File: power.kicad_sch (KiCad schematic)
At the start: 11 parts, among them U3 MAX20356AEWY+T

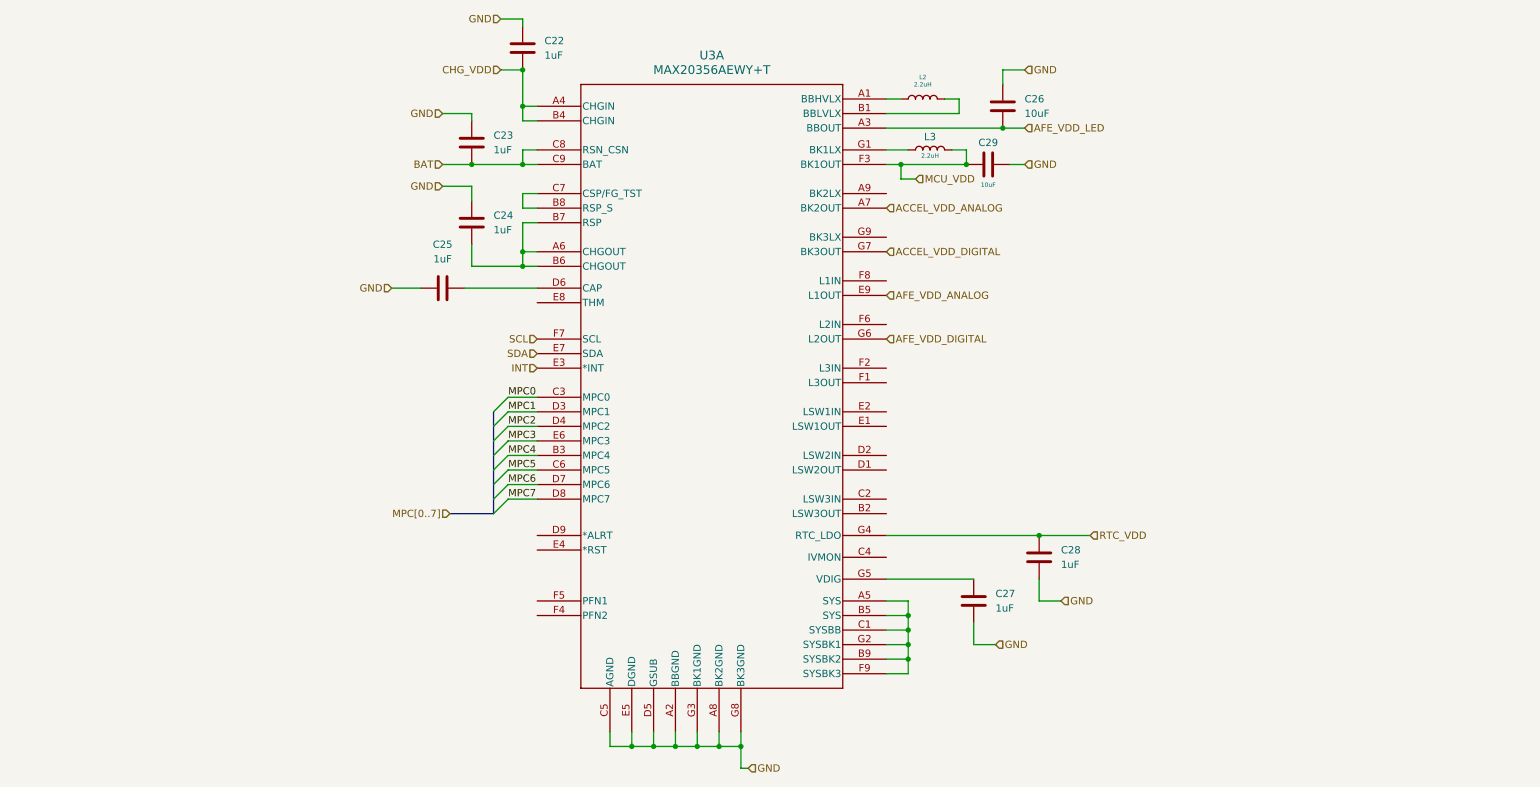
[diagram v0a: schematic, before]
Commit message: inital routing
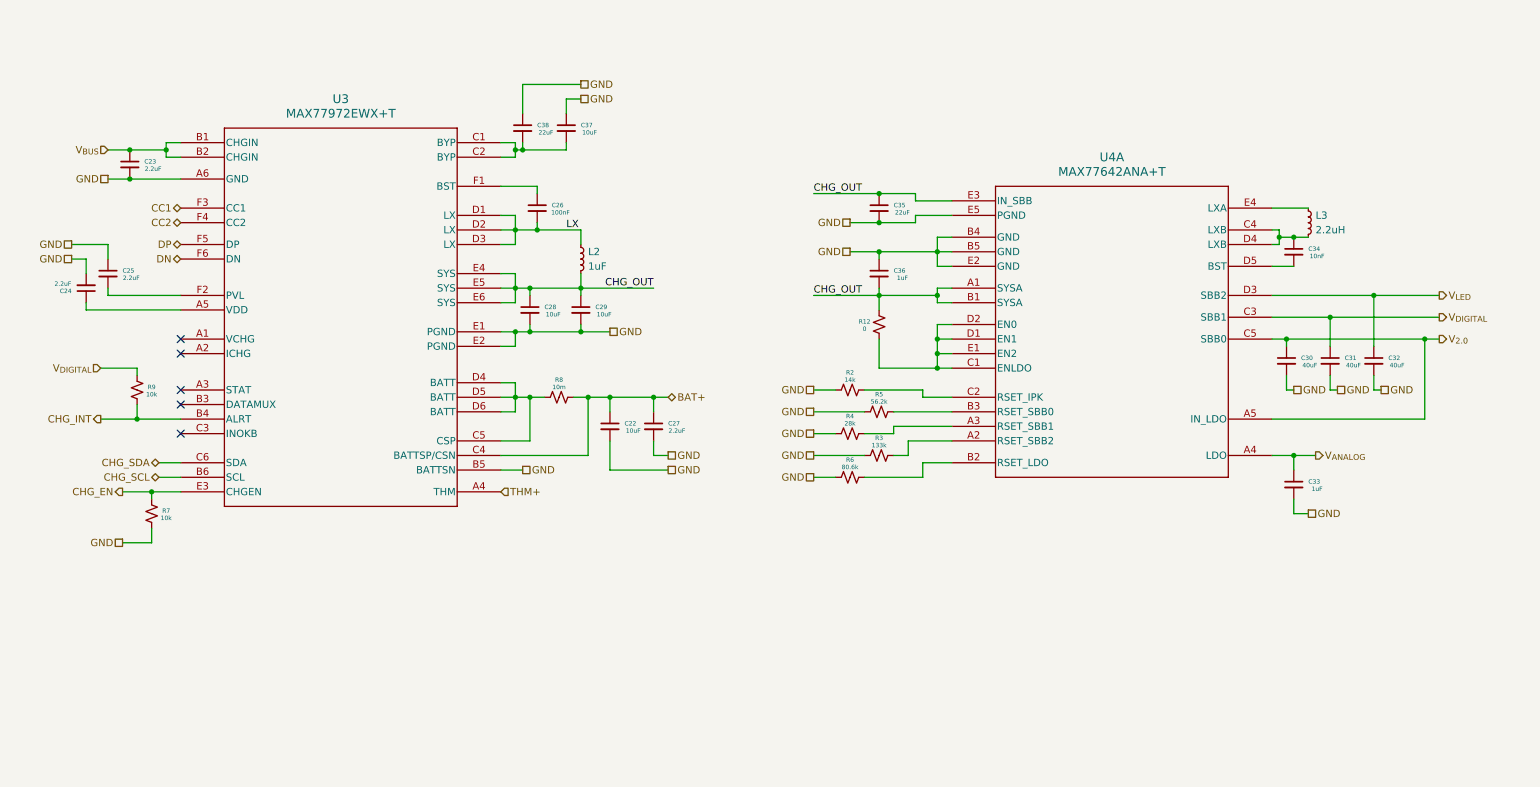
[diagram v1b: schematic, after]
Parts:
- removed C22, C23, C24, C25, C27, C28: 1uF, symbol Device:C
- removed C26, C29: 10uF, symbol Device:C
- removed L2, L3: 2.2uH, symbol Device:L
- removed U3: MAX20356AEWY+T, 21-100616_W633A4+1_ADI, symbol ProjectSymbols:MAX20356AEWY+T
- added C22, C28, C29, C37: 10uF, Capacitor_SMD:C_0402_1005Metric, symbol Device:C_Small
- added C23, C24, C25, C27: 2.2uF, Capacitor_SMD:C_0201_0603Metric, symbol Device:C_Small
- added C26: 100nF, Capacitor_SMD:C_01005_0402Metric, symbol Device:C_Small
- added C30, C31, C32: 40uF, Capacitor_SMD:C_0805_2012Metric, symbol Device:C_Small
- added C33, C36: 1uF, Capacitor_SMD:C_0201_0603Metric, symbol Device:C_Small
- added C34: 10nF, Capacitor_SMD:C_01005_0402Metric, symbol Device:C_Small
- added C35, C38: 22uF, Capacitor_SMD:C_0402_1005Metric, symbol Device:C_Small
- added L2: 1uF, Inductor_SMD:L_0805_2012Metric, symbol Device:L_Small
- added L3: 2.2uH, Inductor_SMD:L_1210_3225Metric, symbol Device:L_Small
- added R12: 0, Resistor_SMD:R_0603_1608Metric, symbol Device:R_Small_US
- added R2: 14k, Resistor_SMD:R_0603_1608Metric, symbol Device:R_Small_US
- added R3: 133k, Resistor_SMD:R_0603_1608Metric, symbol Device:R_Small_US
- added R4: 28k, Resistor_SMD:R_0603_1608Metric, symbol Device:R_Small_US
- added R5: 56.2k, Resistor_SMD:R_0603_1608Metric, symbol Device:R_Small_US
- added R6: 80.6k, Resistor_SMD:R_0603_1608Metric, symbol Device:R_Small_US
- added R7, R9: 10k, Resistor_SMD:R_0603_1608Metric, symbol Device:R_Small_US
- added R8: 10m, Resistor_SMD:R_0603_1608Metric, symbol Device:R_Small_US
- added U3: MAX77972EWX+T, Project-Symbols:MAX77972EWX+T, symbol ProjectSymbols:MAX77972EWX+T
- added U4: MAX77642ANA+T, Project-Symbols:MAX77642ANA+T, symbol ProjectSymbols:MAX77642ANA+T
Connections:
- net GND: now also C22.2, C23.2, C24.2, C25.1, C27.2, C28.2, C29.2, C30.2, C31.2, C32.2, C33.2, C35.2, C36.1, C37.1, C38.1, R2.1, R3.1, R4.1, R5.1, R6.1, R7.2, U3.A6 (GND), U3.B5 (BATTSN), U3.E1 (PGND), U3.E2 (PGND), U4.B4 (GND), U4.B5 (GND), U4.E2 (GND), U4.E5 (PGND)
- new net: R3.2, U4.A2 (RSET_SBB2)
- new net: R12.1, U4.C1 (ENLDO), U4.D1 (EN1), U4.D2 (EN0), U4.E1 (EN2)
- new net: R4.2, U4.A3 (RSET_SBB1)
- new net: R6.2, U4.B2 (RSET_LDO)
- new net: R5.2, U4.B3 (RSET_SBB0)
- new net: R2.2, U4.C2 (RSET_IPK)
- new net: C34.1, L3.2, U4.C4 (LXB), U4.D4 (LXB)
- new net: C34.2, U4.D5 (BST)
- new net: L3.1, U4.E4 (LXA)
- new net: C37.2, C38.2, U3.C1 (BYP), U3.C2 (BYP)
- new net: C26.1, U3.F1 (BST)
- new net: C24.1, U3.A5 (VDD)
- new net: R8.1, U3.C5 (CSP), U3.D4 (BATT), U3.D5 (BATT), U3.D6 (BATT)
- new net: C25.2, U3.F2 (PVL)
- new net BAT+: C22.1, C27.1, R8.2, U3.C4 (BATTSP/CSN)
- new net CC1: U3.F3 (CC1)
- new net CC2: U3.F4 (CC2)
- new net CHG_EN: R7.1, U3.E3 (CHGEN)
- new net CHG_INT: R9.2, U3.B4 (ALRT)
- new net CHG_OUT: C28.1, C29.1, C35.1, C36.2, L2.2, R12.2, U3.E4 (SYS), U3.E5 (SYS), U3.E6 (SYS), U4.A1 (SYSA), U4.B1 (SYSA), U4.E3 (IN_SBB)
- new net CHG_SCL: U3.B6 (SCL)
- new net CHG_SDA: U3.C6 (SDA)
- new net DN: U3.F6 (DN)
- new net DP: U3.F5 (DP)
- new net LX: C26.2, L2.1, U3.D1 (LX), U3.D2 (LX), U3.D3 (LX)
- new net THM+: U3.A4 (THM)
- new net V_{2.0}: C30.1, U4.A5 (IN_LDO), U4.C5 (SBB0)
- new net V_{ANALOG}: C33.1, U4.A4 (LDO)
- new net V_{BUS}: C23.1, U3.B1 (CHGIN), U3.B2 (CHGIN)
- new net V_{DIGITAL}: C31.1, R9.1, U4.C3 (SBB1)
- new net V_{LED}: C32.1, U4.D3 (SBB2)
- no-connect marks 0 -> 5

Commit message: schematic mostly finished
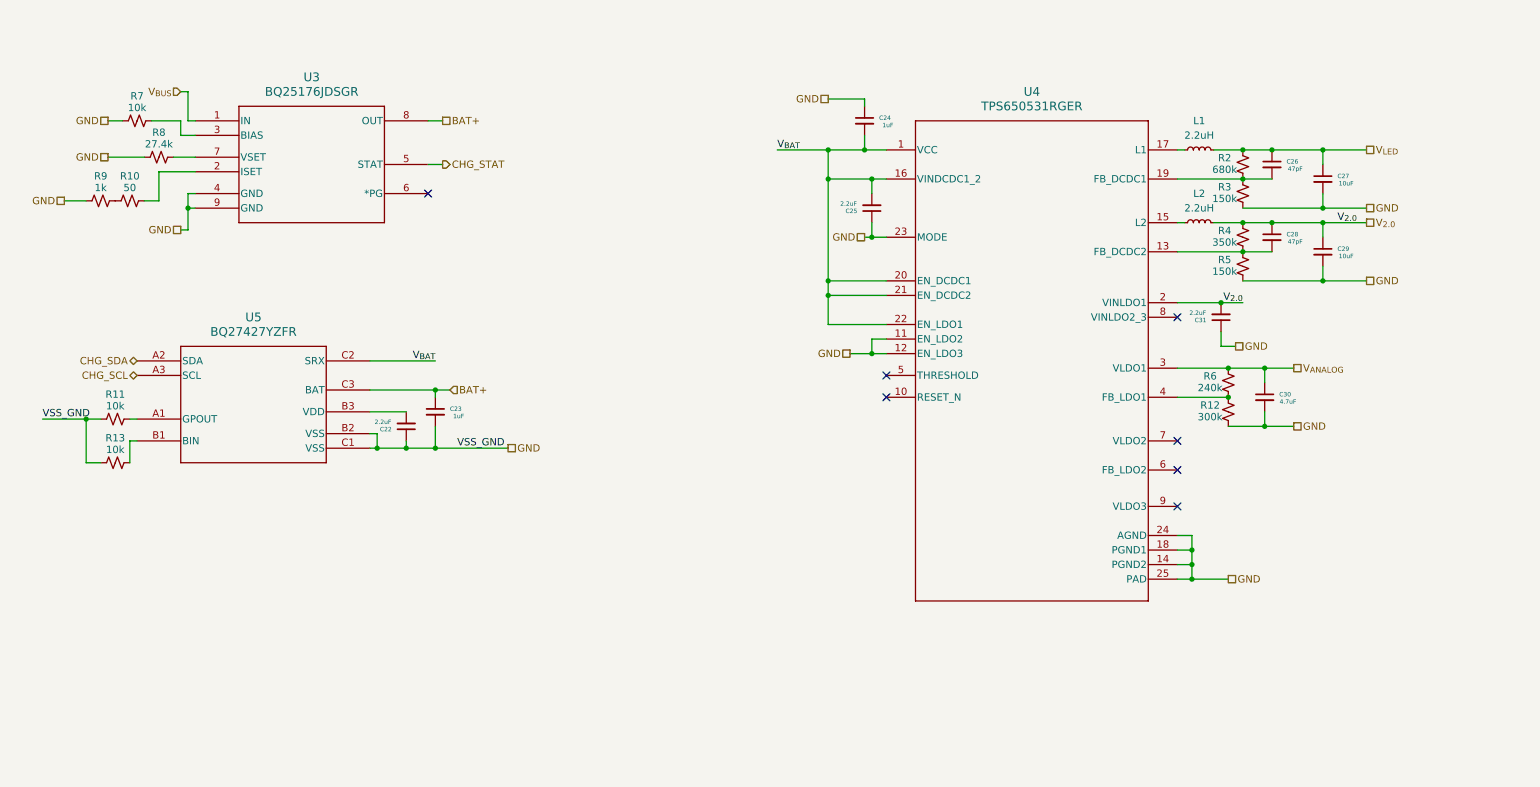
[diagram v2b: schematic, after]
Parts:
- removed C32: 40uF, Capacitor_SMD:C_0805_2012Metric, symbol Device:C_Small
- removed C33, C36: 1uF, Capacitor_SMD:C_0201_0603Metric, symbol Device:C_Small
- removed C34: 10nF, Capacitor_SMD:C_01005_0402Metric, symbol Device:C_Small
- removed C35, C38: 22uF, Capacitor_SMD:C_0402_1005Metric, symbol Device:C_Small
- removed C37: 10uF, Capacitor_SMD:C_0402_1005Metric, symbol Device:C_Small
- removed L3: 2.2uH, Inductor_SMD:L_1210_3225Metric, symbol Device:L_Small
- removed U3: MAX77972EWX+T, Project-Symbols:MAX77972EWX+T, symbol ProjectSymbols:MAX77972EWX+T
- removed U4: MAX77642ANA+T, Project-Symbols:MAX77642ANA+T, symbol ProjectSymbols:MAX77642ANA+T
- added L1: 2.2uH, Inductor_SMD:L_1008_2520Metric, symbol Device:L_Small
- added R10: 50, Resistor_SMD:R_0201_0603Metric, symbol Device:R_Small_US
- added R11, R13: 10k, Resistor_SMD:R_0201_0603Metric, symbol Device:R_Small_US
- added U3: BQ25176JDSGR, Project-Symbols:BQ25176, symbol ProjectSymbols:BQ25176JDSGR
- added U4: TPS650531RGER, Project-Symbols:TPS650531, symbol ProjectSymbols:TPS650531RGER
- added U5: BQ27427YZFR, Project-Symbols:BQ27427, symbol ProjectSymbols:BQ27427YZFR
- C22: value 10uF -> 2.2uF; footprint Capacitor_SMD:C_0402_1005Metric -> Capacitor_SMD:C_0201_0603Metric
- C23, C24: value 2.2uF -> 1uF
- C26: value 100nF -> 47pF
- C27: value 2.2uF -> 10uF
- C28: value 10uF -> 47pF; footprint Capacitor_SMD:C_0402_1005Metric -> Capacitor_SMD:C_01005_0402Metric
- C29: footprint Capacitor_SMD:C_0402_1005Metric -> Capacitor_SMD:C_0201_0603Metric
- C30: value 40uF -> 4.7uF; footprint Capacitor_SMD:C_0805_2012Metric -> Capacitor_SMD:C_0201_0603Metric
- C31: value 40uF -> 2.2uF; footprint Capacitor_SMD:C_0805_2012Metric -> Capacitor_SMD:C_0201_0603Metric
- L2: value 1uF -> 2.2uH; footprint Inductor_SMD:L_0805_2012Metric -> Inductor_SMD:L_1008_2520Metric; MouserURL https://www.mouser.com/ProductDetail/TAIYO-YUDEN/LLEUC2012H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 -> (none)
- R12: value 0 -> 300k; footprint Resistor_SMD:R_0603_1608Metric -> Resistor_SMD:R_0201_0603Metric
- R2: value 14k -> 680k; footprint Resistor_SMD:R_0603_1608Metric -> Resistor_SMD:R_0402_1005Metric_Pad0.72x0.64mm_HandSolder; MouserURL https://www.mouser.com/ProductDetail/Vishay/TNPW060314K0BEE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 -> (none)
- R3: value 133k -> 150k; footprint Resistor_SMD:R_0603_1608Metric -> Resistor_SMD:R_0402_1005Metric_Pad0.72x0.64mm_HandSolder; MouserURL https://www.mouser.com/ProductDetail/Vishay/TNPW060334K0BEE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 -> (none)
- R4: value 28k -> 350k; footprint Resistor_SMD:R_0603_1608Metric -> Resistor_SMD:R_0402_1005Metric_Pad0.72x0.64mm_HandSolder; MouserURL https://www.mouser.com/ProductDetail/Vishay/TNPW060328K0BEE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 -> (none)
- R5: value 56.2k -> 150k; footprint Resistor_SMD:R_0603_1608Metric -> Resistor_SMD:R_0402_1005Metric_Pad0.72x0.64mm_HandSolder; MouserURL https://www.mouser.com/ProductDetail/Vishay/TNPW0603267KBEE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 -> (none)
- R6: value 80.6k -> 240k; footprint Resistor_SMD:R_0603_1608Metric -> Resistor_SMD:R_0201_0603Metric; MouserURL https://www.mouser.com/ProductDetail/Vishay/TNPW060380K6BEE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 -> (none)
- R7: footprint Resistor_SMD:R_0603_1608Metric -> Resistor_SMD:R_0201_0603Metric
- R8: value 10m -> 27.4k; footprint Resistor_SMD:R_0603_1608Metric -> Resistor_SMD:R_0201_0603Metric
- R9: value 10k -> 1k; footprint Resistor_SMD:R_0603_1608Metric -> Resistor_SMD:R_0201_0603Metric
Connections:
- net CHG_EN is gone; now on net GND: R7.1
- net V_{DIGITAL} is gone; now on net GND: C31.1, R9.1
- net BAT+: now also C23.1, U3.8 (OUT), U5.C3 (BAT); no longer C22.1, C27.1, R8.2
- net CHG_SCL: now also U5.A3 (SCL)
- net CHG_SDA: now also U5.A2 (SDA)
- net GND: now also C22.1, C24.1, R12.1, R8.1, R11.1, R13.1, U3.4 (GND), U3.9 (GND), U4.11 (EN_LDO2), U4.12 (EN_LDO3), U4.14 (PGND2), U4.18 (PGND1), U4.23 (MODE), U4.24 (AGND), U4.25 (PAD), U5.B2 (VSS), U5.C1 (VSS); no longer C22.2, C24.2, C28.2, C31.2, R2.1, R4.1, R6.1, R7.2
- net V_{2.0}: now also C28.1, C29.1, C31.2, L2.2, R4.2, U4.2 (VINLDO1); no longer C30.1
- net V_{ANALOG}: now also C30.1, R6.2, U4.3 (VLDO1)
- net V_{BUS}: now also U3.1 (IN); no longer C23.1
- net V_{LED}: now also C26.1, C27.1, R2.2, L1.2
- net at R3.2: now also C26.2, R2.1, U4.19 (FB_DCDC1)
- net at R5.2: now also C28.2, R4.1, U4.13 (FB_DCDC2)
- net V_{BAT}: now reaches C25.2
- net V_{BAT}: now also C24.2, U4.1 (VCC), U4.16 (VINDCDC1_2), U4.20 (EN_DCDC1), U4.21 (EN_DCDC2), U4.22 (EN_LDO1), U5.C2 (SRX)
- net CHG_INT: no longer names the net of R9.2
- net CHG_INT: now also R10.1
- removed net CHG_OUT: C28.1, C29.1, L2.2, R12.2
- net LX: no longer names the net of L2.1
- net LX: now also U4.15 (L2); no longer C26.2
- new net: R7.2, U3.3 (BIAS)
- new net: R10.2, U3.2 (ISET)
- new net: C22.2, U5.B3 (VDD)
- new net: R12.2, R6.1, U4.4 (FB_LDO1)
- new net: R11.2, U5.A1 (GPOUT)
- new net: R13.2, U5.B1 (BIN)
- new net: R8.2, U3.7 (VSET)
- new net: L1.1, U4.17 (L1)
- new net CHG_STAT: U3.5 (STAT)
- no-connect marks 5 -> 7

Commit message: ready to order
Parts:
- C27, C29: footprint Capacitor_SMD:C_0201_0603Metric -> Capacitor_SMD:C_0402_1005Metric
- U3: LCSC PN (none) -> C22407142
- U4: LCSC PN (none) -> C527526
- U5: LSCSC PN (none) -> C6075475
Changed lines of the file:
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@@
 			)
 		)
-		(property "Footprint" "Capacitor_SMD:C_0201_0603Metric"
+		(property "Footprint" "Capacitor_SMD:C_0402_1005Metric"
 			(at 251.46 62.23 0)
 			(effects
@@
 			)
 		)
-		(property "Footprint" "Capacitor_SMD:C_0201_0603Metric"
+		(property "Footprint" "Capacitor_SMD:C_0402_1005Metric"
 			(at 251.46 49.53 0)
 			(effects
@@
 			)
 		)
+		(property "LSCSC PN" "C6075475"
+			(at 44.45 83.82 0)
+			(effects
+				(font
+					(size 1.27 1.27)
+				)
+				(hide yes)
+			)
+		)
 		(pin "C1"
 		)
@@
 			)
 		)
+		(property "LCSC PN" "C22407142"
+			(at 54.61 41.91 0)
+			(effects
+				(font
+					(size 1.27 1.27)
+				)
+				(hide yes)
+			)
+		)
 		(pin "3"
 		)
@@
 			(at 200.66 90.17 0)
 			(effects
+				(font
+					(size 1.27 1.27)
+				)
+				(hide yes)
+			)
+		)
+		(property "LCSC PN" "C527526"
+			(at 200.66 90.17 0)
+			(effects

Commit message: resize to 0603
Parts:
- C22, C23, C24, C25, C30, C31: footprint Capacitor_SMD:C_0201_0603Metric -> Capacitor_SMD:C_0603_1608Metric
- C26, C28: footprint Capacitor_SMD:C_01005_0402Metric -> Capacitor_SMD:C_0603_1608Metric
- C27, C29: footprint Capacitor_SMD:C_0402_1005Metric -> Capacitor_SMD:C_0603_1608Metric
- R10, R11, R12, R13, R6, R7, R8, R9: footprint Resistor_SMD:R_0201_0603Metric -> Resistor_SMD:R_0603_1608Metric
- R2, R3, R4, R5: footprint Resistor_SMD:R_0402_1005Metric_Pad0.72x0.64mm_HandSolder -> Resistor_SMD:R_0603_1608Metric
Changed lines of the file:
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@@
 			)
 		)
-		(property "Footprint" "Resistor_SMD:R_0201_0603Metric"
+		(property "Footprint" "Resistor_SMD:R_0603_1608Metric"
 			(at 44.45 39.37 0)
 			(effects
@@
 			)
 		)
-		(property "Footprint" "Capacitor_SMD:C_0402_1005Metric"
+		(property "Footprint" "Capacitor_SMD:C_0603_1608Metric"
 			(at 251.46 62.23 0)
 			(effects
@@
 			)
 		)
-		(property "Footprint" "Resistor_SMD:R_0402_1005Metric_Pad0.72x0.64mm_HandSolder"
+		(property "Footprint" "Resistor_SMD:R_0603_1608Metric"
 			(at 237.49 64.77 0)
 			(effects
@@
 			)
 		)
-		(property "Footprint" "Resistor_SMD:R_0402_1005Metric_Pad0.72x0.64mm_HandSolder"
+		(property "Footprint" "Resistor_SMD:R_0603_1608Metric"
 			(at 237.49 46.99 0)
 			(effects
@@
 			)
 		)
-		(property "Footprint" "Resistor_SMD:R_0201_0603Metric"
+		(property "Footprint" "Resistor_SMD:R_0603_1608Metric"
 			(at 43.18 53.34 0)
 			(effects
@@
 			)
 		)
-		(property "Footprint" "Resistor_SMD:R_0402_1005Metric_Pad0.72x0.64mm_HandSolder"
+		(property "Footprint" "Resistor_SMD:R_0603_1608Metric"
 			(at 237.49 52.07 0)
 			(effects
@@
 			)
 		)
-		(property "Footprint" "Capacitor_SMD:C_0201_0603Metric"
+		(property "Footprint" "Capacitor_SMD:C_0603_1608Metric"
 			(at 233.68 73.66 0)
 			(effects
@@
 			)
 		)
-		(property "Footprint" "Capacitor_SMD:C_0201_0603Metric"
+		(property "Footprint" "Capacitor_SMD:C_0603_1608Metric"
 			(at 91.44 92.71 0)
 			(effects
@@
 			)
 		)
-		(property "Footprint" "Capacitor_SMD:C_0402_1005Metric"
+		(property "Footprint" "Capacitor_SMD:C_0603_1608Metric"
 			(at 251.46 49.53 0)
 			(effects
@@
 			)
 		)
-		(property "Footprint" "Resistor_SMD:R_0201_0603Metric"
+		(property "Footprint" "Resistor_SMD:R_0603_1608Metric"
 			(at 234.95 85.09 0)
 			(effects
@@
 			)
 		)
-		(property "Footprint" "Capacitor_SMD:C_0201_0603Metric"
+		(property "Footprint" "Capacitor_SMD:C_0603_1608Metric"
 			(at 171.45 39.37 0)
 			(effects
@@
 			)
 		)
-		(property "Footprint" "Resistor_SMD:R_0201_0603Metric"
+		(property "Footprint" "Resistor_SMD:R_0603_1608Metric"
 			(at 40.64 99.06 0)
 			(effects
@@
 			)
 		)
-		(property "Footprint" "Resistor_SMD:R_0402_1005Metric_Pad0.72x0.64mm_HandSolder"
+		(property "Footprint" "Resistor_SMD:R_0603_1608Metric"
 			(at 237.49 59.69 0)
 			(effects
@@
 			)
 		)
-		(property "Footprint" "Capacitor_SMD:C_0201_0603Metric"
+		(property "Footprint" "Capacitor_SMD:C_0603_1608Metric"
 			(at 172.72 54.61 0)
 			(effects
@@
 			)
 		)
-		(property "Footprint" "Capacitor_SMD:C_0201_0603Metric"
+		(property "Footprint" "Capacitor_SMD:C_0603_1608Metric"
 			(at 96.52 90.17 0)
 			(effects
@@
 			)
 		)
-		(property "Footprint" "Resistor_SMD:R_0201_0603Metric"
+		(property "Footprint" "Resistor_SMD:R_0603_1608Metric"
 			(at 234.95 90.17 0)
 			(effects
@@
 			)
 		)
-		(property "Footprint" "Resistor_SMD:R_0201_0603Metric"
+		(property "Footprint" "Resistor_SMD:R_0603_1608Metric"
 			(at 48.26 45.72 0)
 			(effects
@@
 			)
 		)
-		(property "Footprint" "Resistor_SMD:R_0201_0603Metric"
+		(property "Footprint" "Resistor_SMD:R_0603_1608Metric"
 			(at 38.1 53.34 0)
 			(effects
@@
 			)
 		)
-		(property "Footprint" "Resistor_SMD:R_0201_0603Metric"
+		(property "Footprint" "Resistor_SMD:R_0603_1608Metric"
 			(at 40.64 91.44 0)
 			(effects
@@
 			)
 		)
-		(property "Footprint" "Capacitor_SMD:C_01005_0402Metric"
+		(property "Footprint" "Capacitor_SMD:C_0603_1608Metric"
 			(at 242.57 59.69 0)
 			(effects
@@
 			)
 		)
-		(property "Footprint" "Capacitor_SMD:C_0201_0603Metric"
+		(property "Footprint" "Capacitor_SMD:C_0603_1608Metric"
 			(at 241.3 87.63 0)
 			(effects
@@
 			)
 		)
-		(property "Footprint" "Capacitor_SMD:C_01005_0402Metric"
+		(property "Footprint" "Capacitor_SMD:C_0603_1608Metric"
 			(at 242.57 46.99 0)
 			(effects

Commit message: final order
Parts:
- L1, L2: LCSC PN (none) -> C23894
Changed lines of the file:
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@@
+			)
+		)
+		(property "LCSC PN" "C23894"
+			(at 229.87 57.15 90)
+			(effects
+				(font
+					(size 1.27 1.27)
+				)
+				(hide yes)
 			)
 		)
@@
 			(effects
 				(font
+					(size 1.27 1.27)
+				)
+				(hide yes)
+			)
+		)
+		(property "LCSC PN" "C23894"
+			(at 229.87 44.45 90)
+			(effects
+				(font
